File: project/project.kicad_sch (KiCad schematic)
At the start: 30 parts, among them J1 Conn_02x16_Odd_Even, J2 TYPE-C 6P(040新), SW1 SS-12D10L9, U1 DRV8833PWPR, U2 CH224K, U3 DRV8833PWPR, U4 AP63203WU-7, U5 TP4056

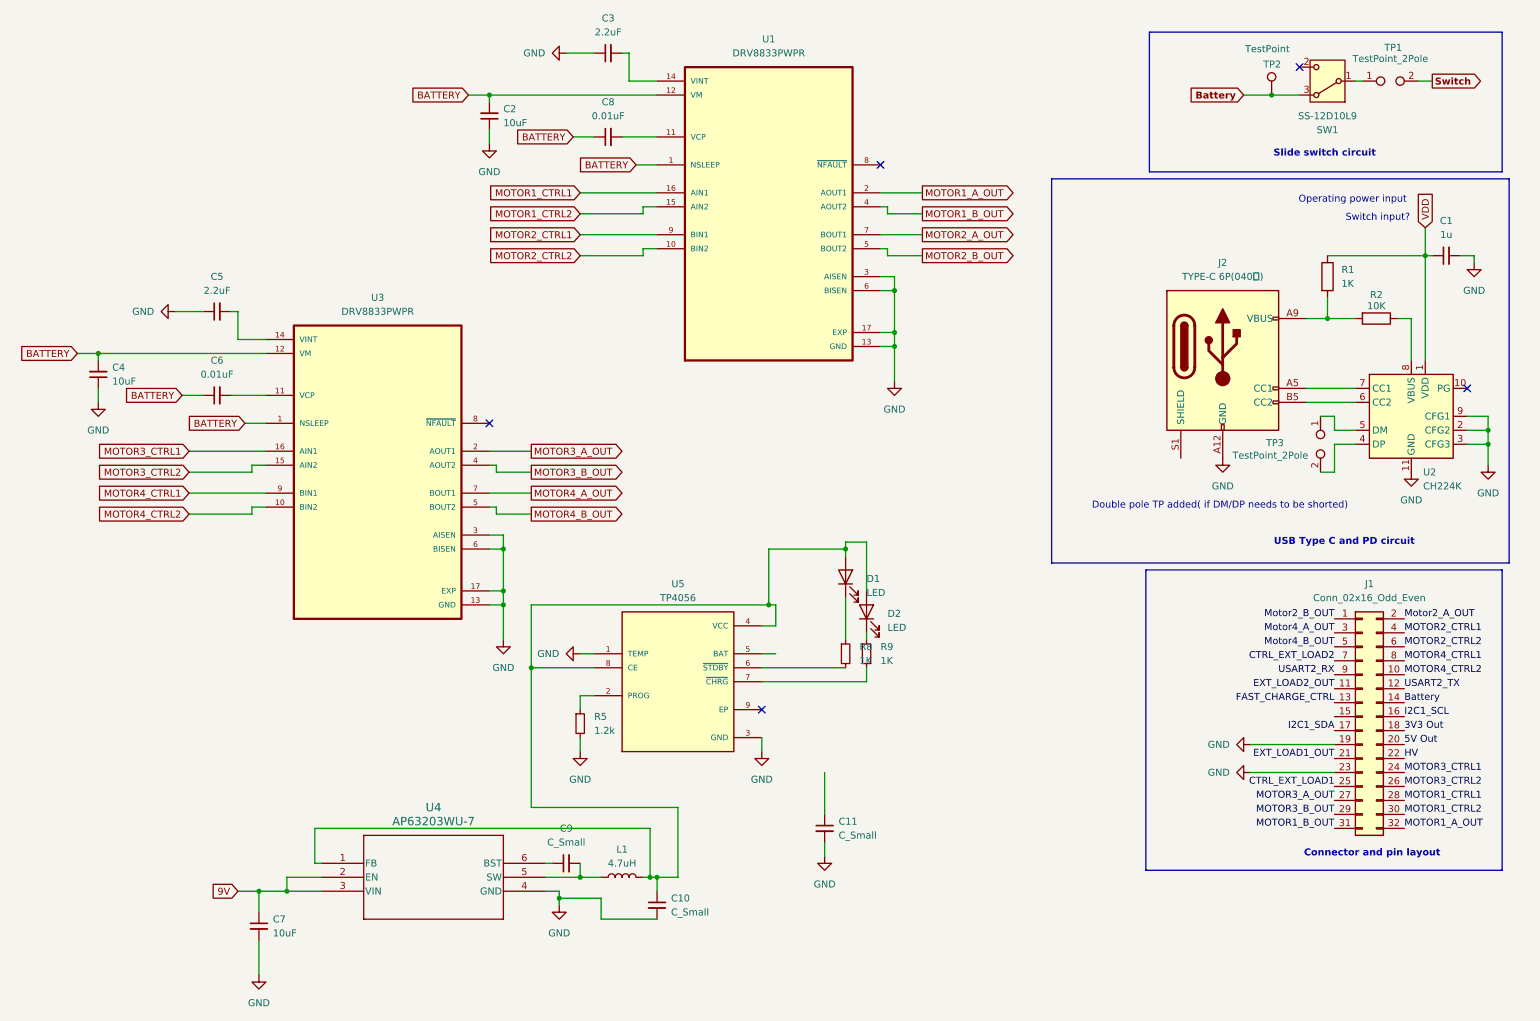
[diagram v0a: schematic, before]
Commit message: Rearranged.
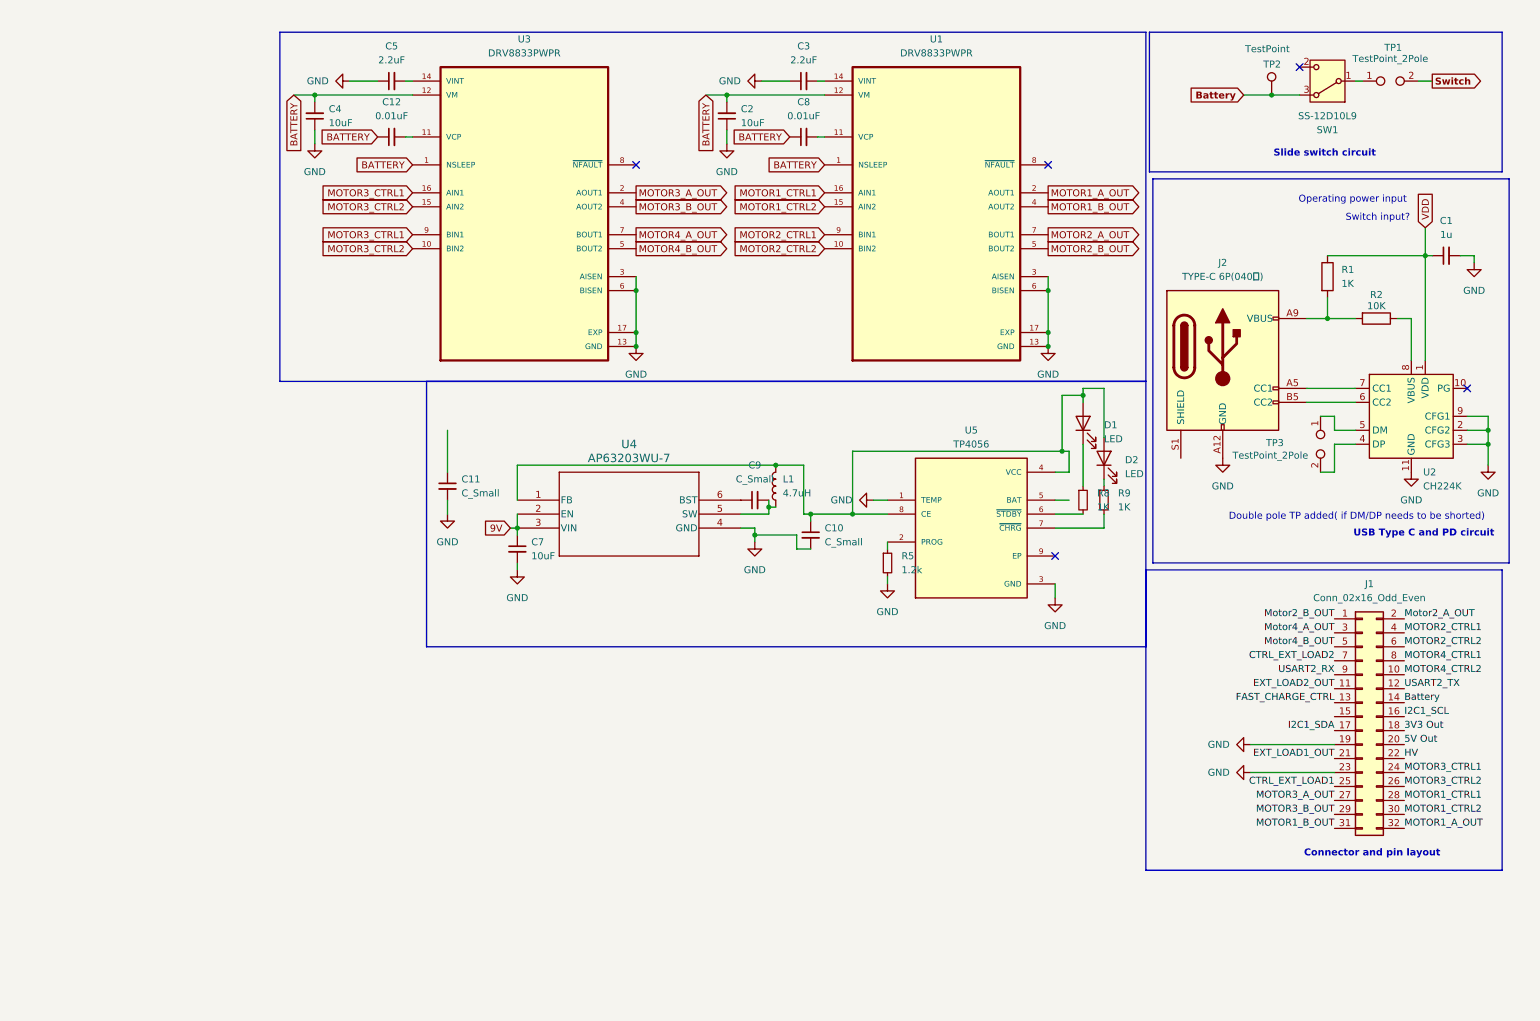
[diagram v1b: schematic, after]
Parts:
- removed C6: 0.01uF, symbol Device:C_Small
- added C12: 0.01uF, symbol Device:C_Small
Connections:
- net BATTERY: now also C12.1
- net MOTOR3_CTRL1: now also U3.9 (BIN1)
- net MOTOR3_CTRL2: now also U3.10 (BIN2)
- net MOTOR4_CTRL1: no longer U3.9 (BIN1)
- net MOTOR4_CTRL2: no longer U3.10 (BIN2)
- net at U3.11 (VCP): now also C12.2
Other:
- moved on the sheet: C10, C11, C2, C3, C7, C8, C9, D1, D2, L1, R5, R8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
